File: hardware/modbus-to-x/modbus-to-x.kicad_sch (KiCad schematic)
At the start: 33 parts, among them J1 PWR, J2 UART, SW1 SW_Push, SW2 SW_Push, U1 AMS1117-3.3, U3 MAX3485, U4 ESP32-WROOM-32D, U5 AT24CS64-XHM, U6 AT24CS64-XHM, U7 LMR14020SQDPRTQ1

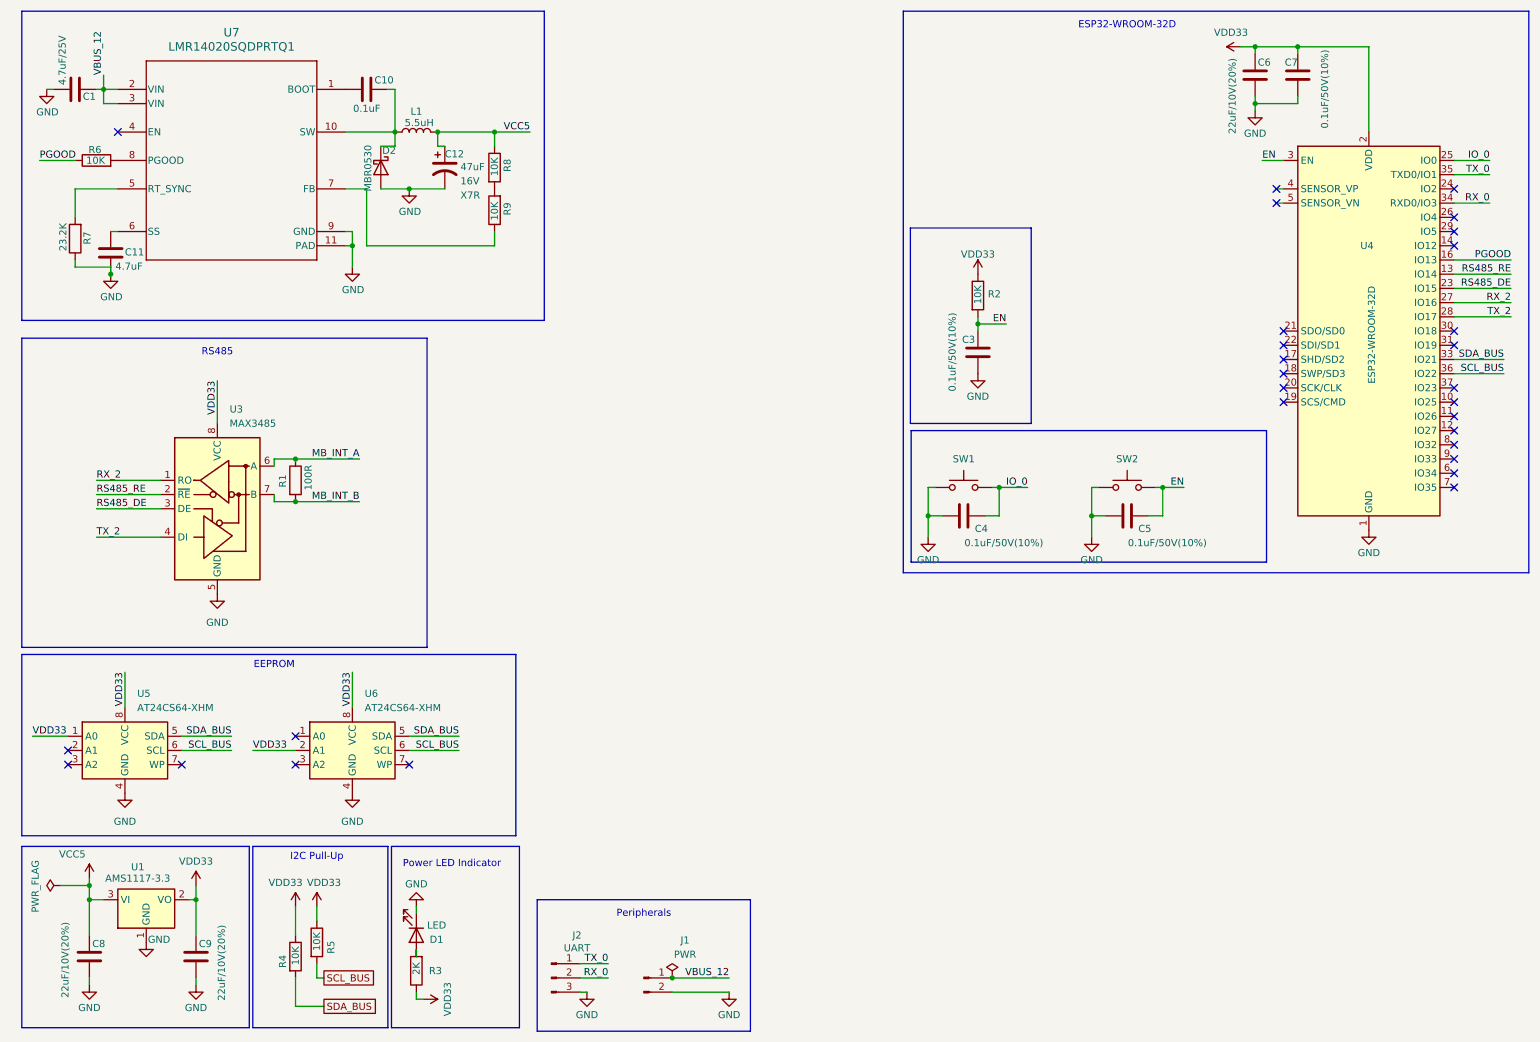
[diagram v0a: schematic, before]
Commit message: updated hw
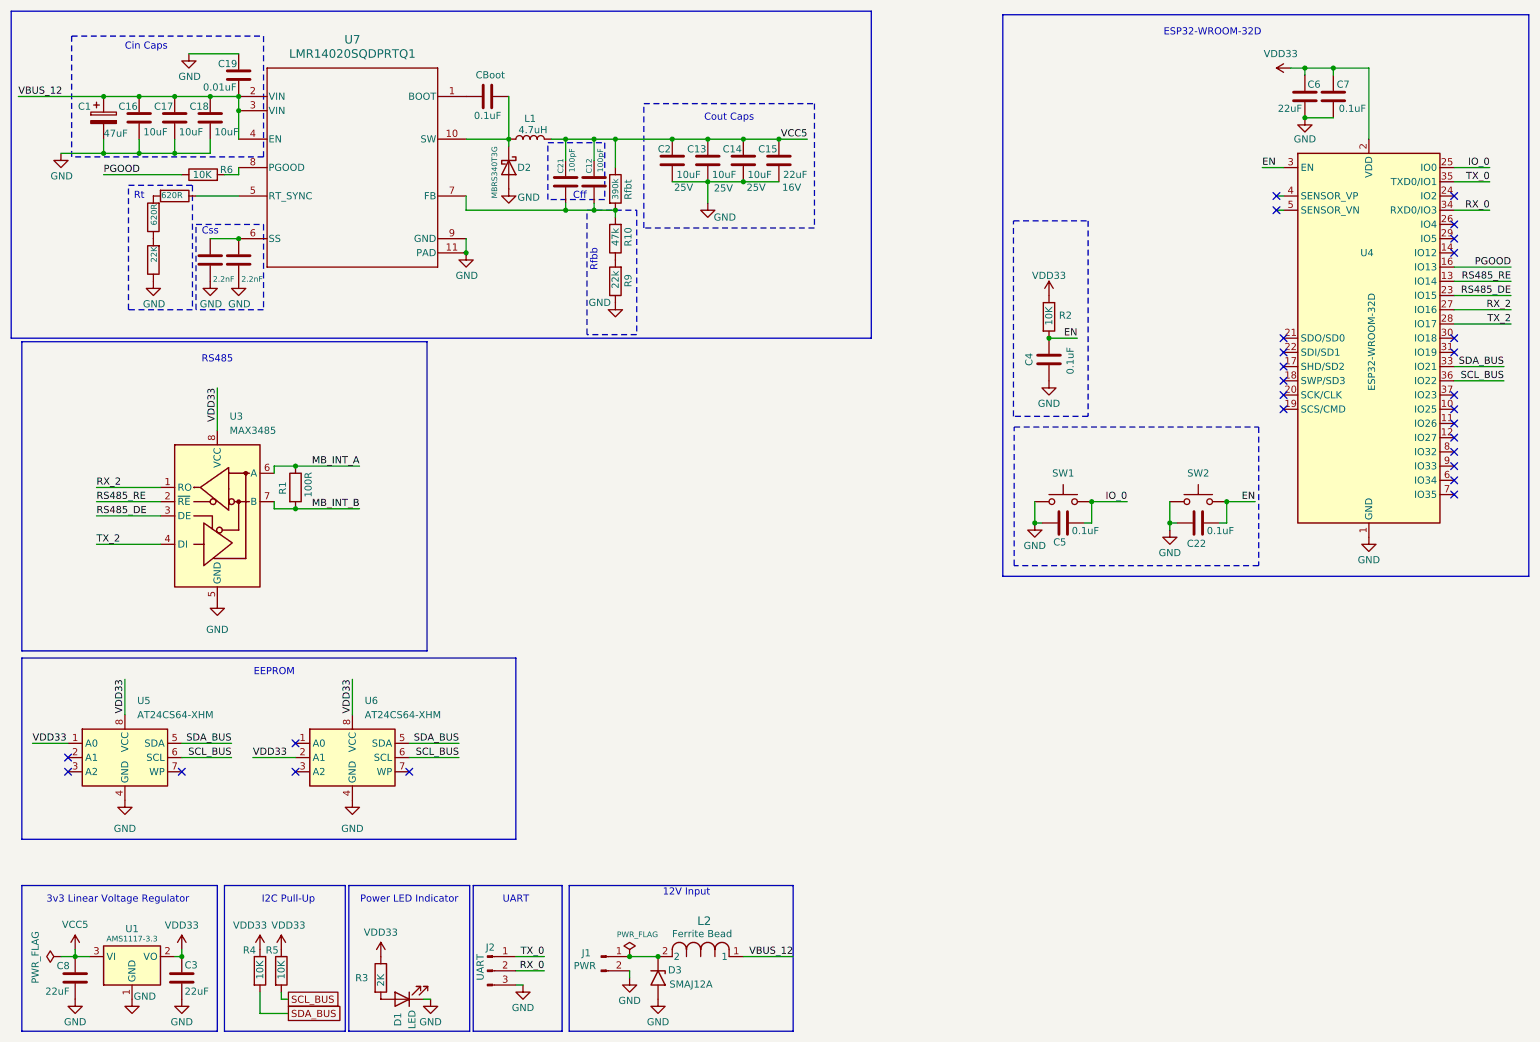
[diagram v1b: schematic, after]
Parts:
- removed C1: 4.7uF/25V, Capacitor_SMD:C_0805_2012Metric_Pad1.18x1.45mm_HandSolder, symbol Device:C
- removed C12: 47uF, ~, symbol SparkFun-Capacitor:C_Polarized
- removed C9: 22uF/10V(20%), Capacitor_SMD:C_0402_1005Metric_Pad0.74x0.62mm_HandSolder, symbol Device:C
- added C1: 47uF, Capacitor_SMD:CP_Elec_6.3x5.4, symbol Device:C_Polarized
- added C12, C21: 100pF, Capacitor_SMD:C_0805_2012Metric_Pad1.18x1.45mm_HandSolder, symbol Device:C
- added C13, C14, C16, C17, C18, C2: 10uF, Capacitor_SMD:C_0805_2012Metric_Pad1.18x1.45mm_HandSolder, symbol Device:C
- added C15: 22uF, Capacitor_SMD:C_0805_2012Metric_Pad1.18x1.45mm_HandSolder, symbol Device:C
- added C19: 0.01uF, Capacitor_SMD:C_0402_1005Metric_Pad0.74x0.62mm_HandSolder, symbol Device:C
- added C20: 2.2nF, Capacitor_SMD:C_0805_2012Metric_Pad1.18x1.45mm_HandSolder, symbol Device:C
- added C22: 0.1uF, Capacitor_SMD:C_1206_3216Metric_Pad1.33x1.80mm_HandSolder, symbol Device:C
- added D3: SMAJ12A, Diode_SMD:D_SMA_Handsoldering, symbol Diode:SMAJ12A
- added L2: MPZ1005S121CT000, MPZ1005S121CT000:IND_1005_TDK-L, symbol MPZ1005S121CT000:MPZ1005S121CT000
- added R10: 47k, Resistor_SMD:R_0805_2012Metric_Pad1.20x1.40mm_HandSolder, symbol Device:R
- added R11: 22K, Resistor_SMD:R_0603_1608Metric_Pad0.98x0.95mm_HandSolder, symbol Device:R
- added R12: 620R, Resistor_SMD:R_0805_2012Metric_Pad1.20x1.40mm_HandSolder, symbol Device:R
- C10: FriendlyName (none) -> CBoot; PartNo (none) -> CC0402MRX5R7BB104; Voltage (none) -> 16V
- C11: value 4.7uF -> 2.2nF; footprint Capacitor_SMD:C_0402_1005Metric_Pad0.74x0.62mm_HandSolder -> Capacitor_SMD:C_0805_2012Metric_Pad1.18x1.45mm_HandSolder; FriendlyName (none) -> Css; PartNo (none) -> RND 1500805B222J500NT; Voltage (none) -> 50V
- C3: value 0.1uF/50V(10%) -> 22uF; footprint Capacitor_SMD:C_0402_1005Metric_Pad0.74x0.62mm_HandSolder -> Capacitor_SMD:C_0805_2012Metric_Pad1.18x1.45mm_HandSolder; ProductCode (none) -> CL21A226MOCLRNC; now left out of the parts list
- C4, C5, C7: value 0.1uF/50V(10%) -> 0.1uF; footprint Capacitor_SMD:C_0402_1005Metric_Pad0.74x0.62mm_HandSolder -> Capacitor_SMD:C_1206_3216Metric_Pad1.33x1.80mm_HandSolder; ProductCode (none) -> CVNF100K12X; now left out of the parts list
- C6, C8: value 22uF/10V(20%) -> 22uF; footprint Capacitor_SMD:C_0402_1005Metric_Pad0.74x0.62mm_HandSolder -> Capacitor_SMD:C_0805_2012Metric_Pad1.18x1.45mm_HandSolder; ProductCode (none) -> CL21A226MOCLRNC; now left out of the parts list
- D1, J1, J2, R2, R3, R4, R5, SW1, SW2, U1, U3, U4, U5, U6: now left out of the parts list
- D2: value MBR0530 -> MBRS340T3G; footprint Diode_SMD:D_SOD-123 -> Diode_SMD:D_SMB-SMC_Universal_Handsoldering; PartNo (none) -> MBRS340T3G
- L1: value 5.5uH -> 4.7uH; footprint SparkFun-Capacitor:C_0805_2012Metric -> WE 74404041047:L_Wurth_WE-LQS-4012; PROD_ID NDUC- -> (none); PartNo (none) -> WE 74404041047
- R1: footprint (none) -> Resistor_SMD:R_1206_3216Metric_Pad1.30x1.75mm_HandSolder; ProductCode (none) -> 1551206S4F1000T5E; now left out of the parts list
- R6: PartNo (none) -> 155TC0525B1002T5J
- R7: value 23.2K -> 620R; FriendlyName (none) -> Rt; PartNo (none) -> 1550805S8F6200T5E
- R8: value 10K -> 390k; footprint Resistor_SMD:R_0805_2012Metric_Pad1.20x1.40mm_HandSolder -> Resistor_SMD:R_0402_1005Metric_Pad0.72x0.64mm_HandSolder; FriendlyName (none) -> Rfbt
- R9: value 10K -> 22k; footprint Resistor_SMD:R_0805_2012Metric_Pad1.20x1.40mm_HandSolder -> Resistor_SMD:R_0603_1608Metric_Pad0.98x0.95mm_HandSolder; FriendlyName (none) -> Rfbb2
- U7: footprint DPR0010A -> LMR14020SQDPRTQ1:DPR0010A
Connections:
- net EN: now also C4.1, C22.1; no longer C3.2, C5.2
- net GND: now also C3.2, C4.2, C5.2, R9.1, C1.2, C13.1, C14.1, C15.1, C16.1, C17.1, C18.1, C19.2, C2.1, C20.1, C22.2, D3.2 (A2), R11.1; no longer C3.1, C4.1, C5.1, R7.1
- net IO_0: now also C5.1; no longer C4.2
- net VBUS_12: now also U7.4 (EN), C1.1, C16.2, C17.2, C18.2, C19.1, L2.1; no longer J1.1 (Pin_1)
- net VCC5: now also C12.2, C13.2, C14.2, C15.2, C2.2, C21.2
- net VDD33: now also C3.1
- net at U7.5 (RT_SYNC): now also R12.1; no longer R7.2
- net at C11.2, U7.6 (SS): now also C20.2
- net at U7.7 (FB): now also R8.2, C12.1, C21.1, R10.2; no longer R9.1
- net at R9.2: now also R10.1; no longer R8.2
- new net: D3.1 (A1), J1.1 (Pin_1), L2.2
- new net: R12.2, R7.2
- new net: R11.2, R7.1
- no-connect marks 29 -> 28
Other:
- note added: "12V Input"
- note added: "3v3 Linear Voltage Regulator"
- note added: "Cff"
- note added: "Cin Caps"
- note added: "Cout Caps"
- note added: "Css"
- note added: "Rfbb"
- note added: "Rt"
- note added: "UART"
- note removed: "Peripherals"
- moved on the sheet: C6, C7, C8, D1, D2, J1, J2, L1, R1, R2, R3, R4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
